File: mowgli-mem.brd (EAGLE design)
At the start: 80.6 x 23.9 mm, 23 parts, among them IC1 ATMEGA, IC2 MCP1702-33, IC3 AT24CP, IC4 DS1307, Q1 32.768, X1 16 MHz, X3 JSTPH

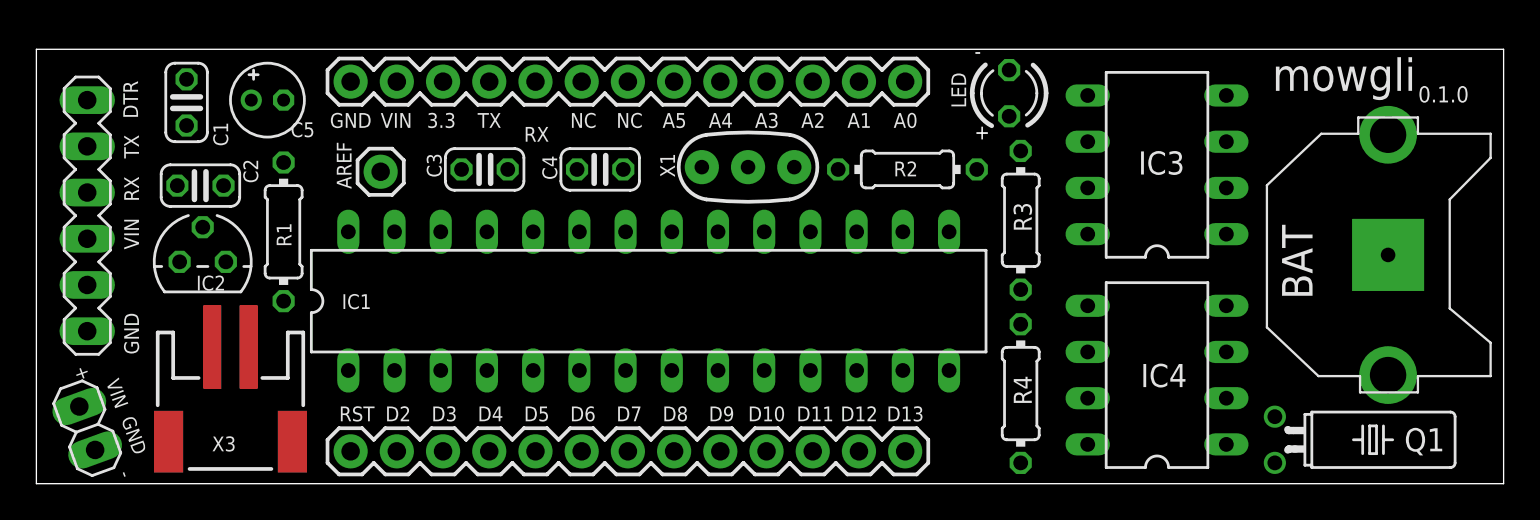
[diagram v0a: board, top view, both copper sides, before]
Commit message: update
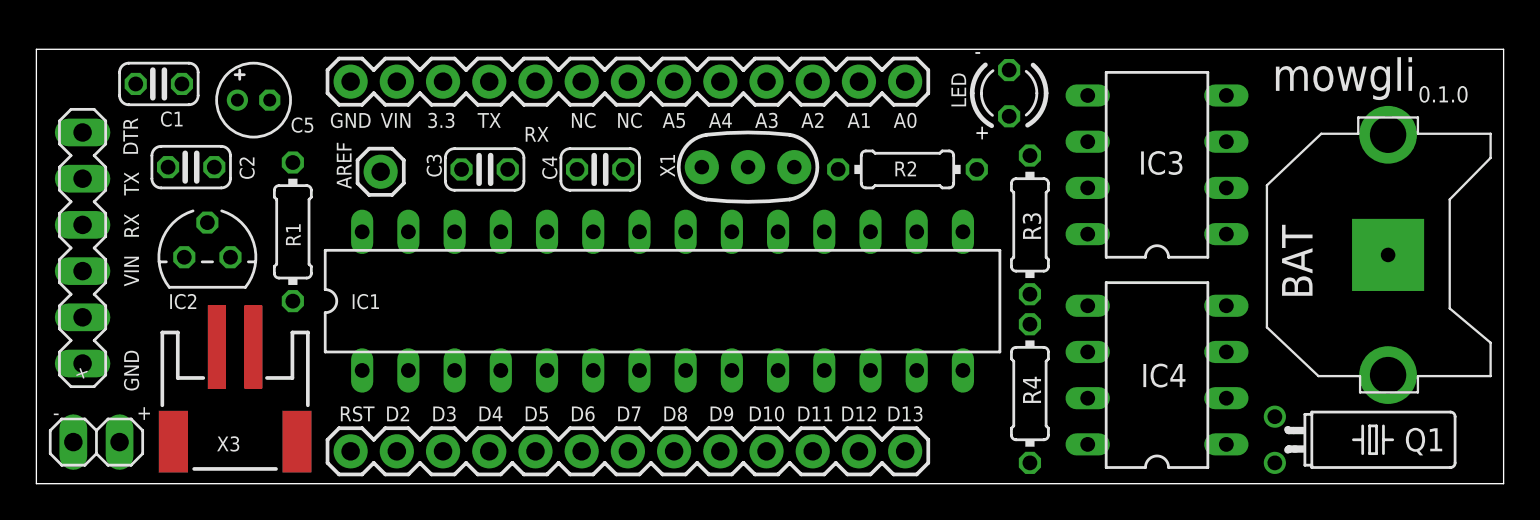
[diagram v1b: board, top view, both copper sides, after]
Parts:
- moved C1 1.83 mm to (5.97, 21.5), turned to 180 degrees
- moved FTDI 1.80 mm to (1.78, 6.10)
- moved C2 1.14 mm to (7.75, 16.9)
- moved JP1 0.92 mm to (2.54, 1.78), turned to 180 degrees
- moved C5 0.76 mm to (11.2, 20.6)
- moved IC1 0.76 mm to (33.7, 9.53)
- moved R3 0.57 mm to (53.8, 13.7)
- moved R1 0.51 mm to (13.3, 13.3)
- moved R4 0.51 mm to (53.8, 4.45)
- moved IC2 0.36 mm to (8.64, 11.9)
- moved X3 0.25 mm to (10.2, 3.30)
